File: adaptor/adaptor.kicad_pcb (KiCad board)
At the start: 2 copper layers, 37.6 x 23.6 mm, 7 parts, among them J1 1-84952-5, J2 1-84952-5

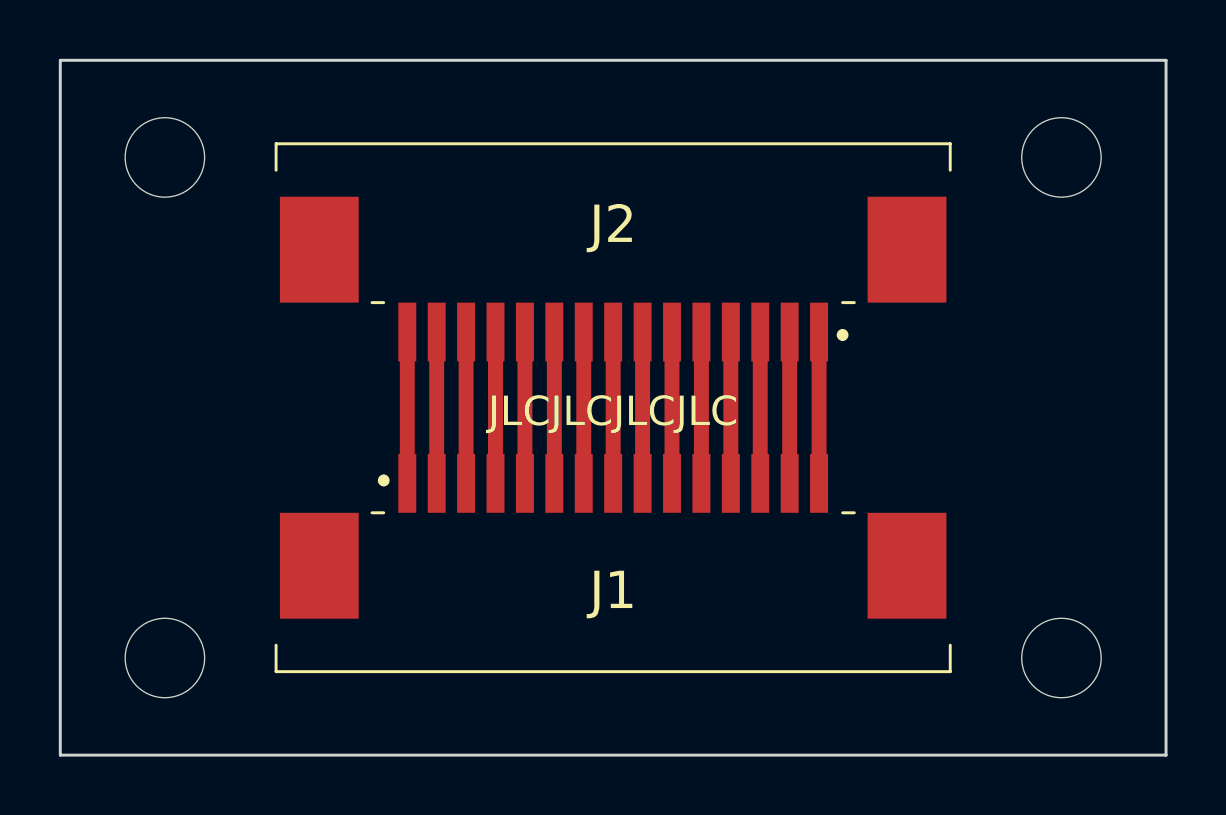
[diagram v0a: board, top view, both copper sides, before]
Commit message: model & add break off board tommorow
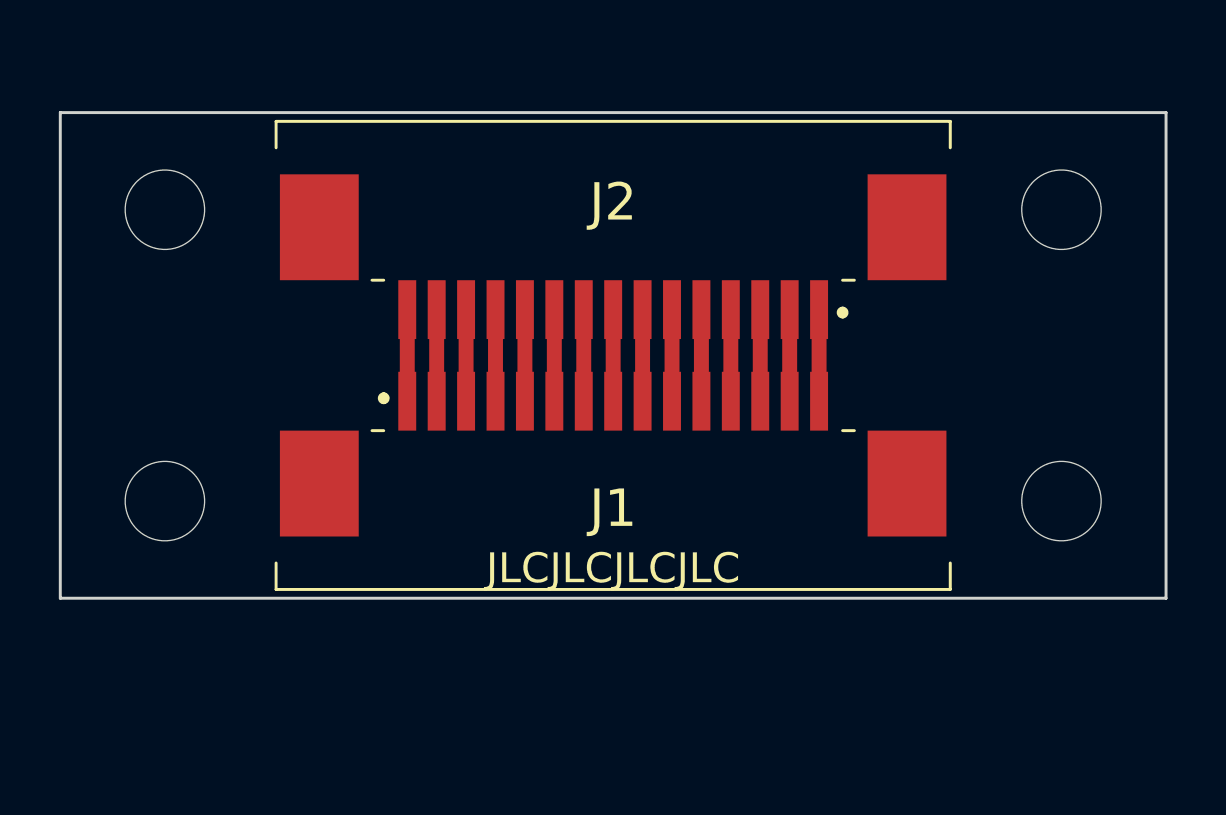
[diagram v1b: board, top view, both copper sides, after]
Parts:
- removed the REF** at (126.7, 114.0)
- moved REF** 5.33 mm to (142.0, 112.3)
- moved REF** 5.33 mm to (111.5, 112.3)
- moved J1 2.79 mm to (126.7, 112.5)
- moved REF** 1.78 mm to (142.0, 102.4)
- moved REF** 1.78 mm to (111.5, 102.4)
- moved J2 0.76 mm to (126.7, 102.1)
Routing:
- net Net-(J1-Pad9): track 5.15 -> 3.37 mm
- net Net-(J1-Pad8): track 5.15 -> 3.37 mm
- net Net-(J1-Pad7): track 5.15 -> 3.37 mm
- net Net-(J1-Pad6): track 5.15 -> 3.37 mm
- net Net-(J1-Pad5): track 5.15 -> 3.37 mm
- net Net-(J1-Pad4): track 5.15 -> 3.37 mm
- net Net-(J1-Pad3): track 5.15 -> 3.37 mm
- net Net-(J1-Pad2): track 5.15 -> 3.37 mm
- net Net-(J1-Pad15): track 5.15 -> 3.37 mm
- net Net-(J1-Pad14): track 5.15 -> 3.37 mm
- net Net-(J1-Pad13): track 5.15 -> 3.37 mm
- net Net-(J1-Pad12): track 5.15 -> 3.37 mm
- net Net-(J1-Pad11): track 5.15 -> 3.37 mm
- net Net-(J1-Pad10): track 5.15 -> 3.37 mm
- net Net-(J1-Pad1): track 5.15 -> 3.37 mm
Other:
- board size 37.6 x 23.6 mm -> 37.6 x 16.5 mm
